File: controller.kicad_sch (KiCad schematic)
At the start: 14 parts, among them J1 Conn_01x06_Female, J2 Conn_01x06_Female, J3 Conn_01x022_Male

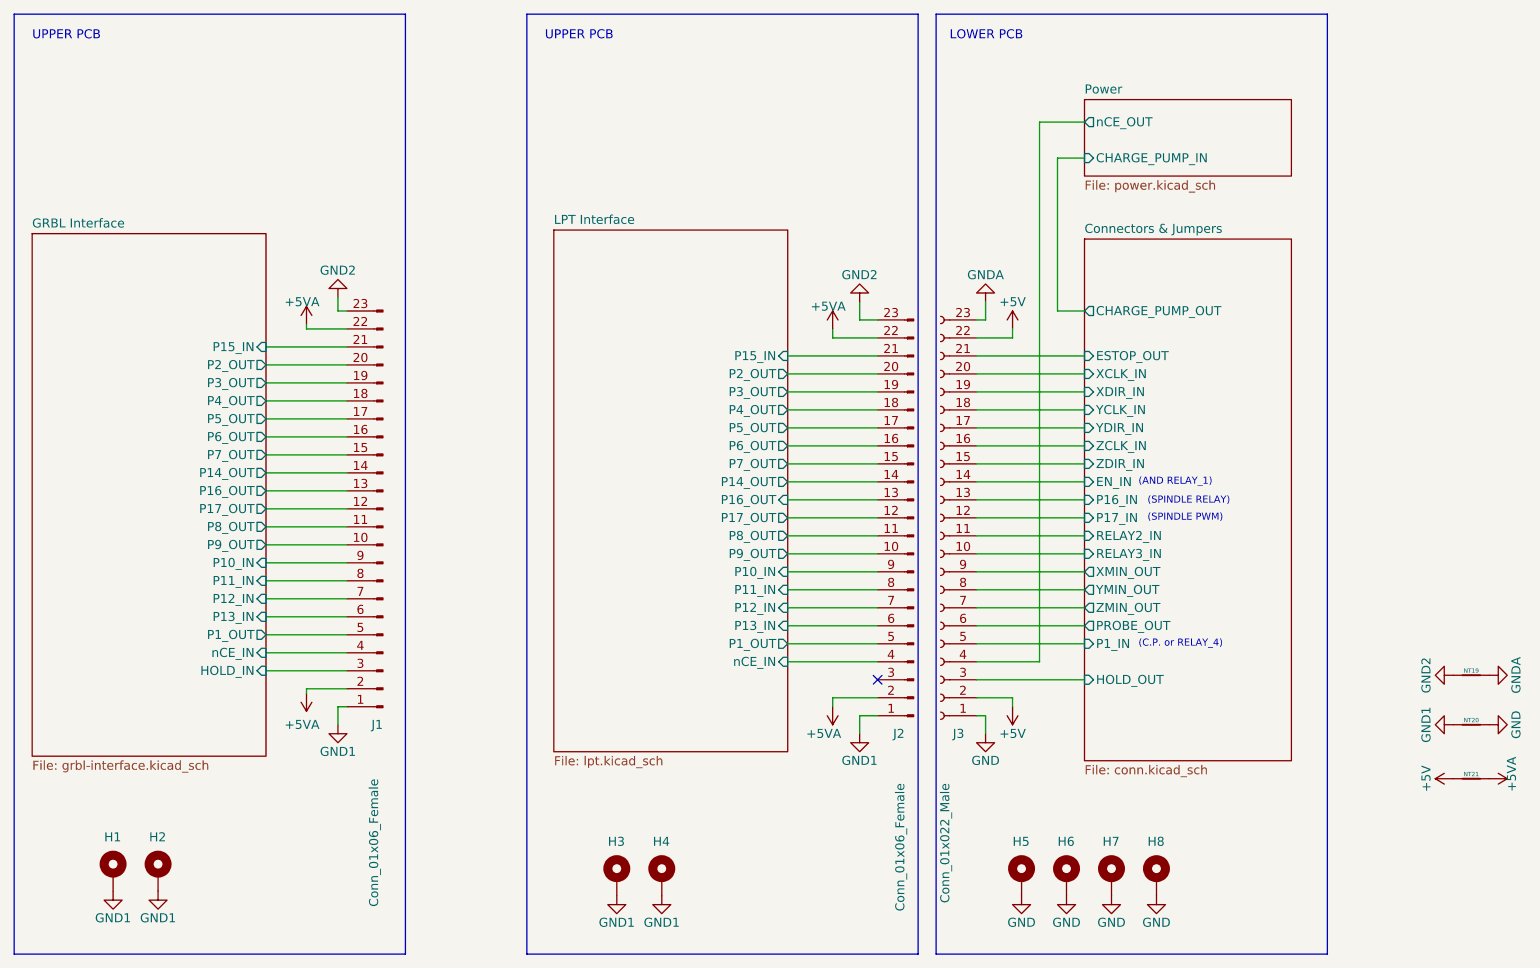
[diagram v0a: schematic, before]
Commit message: GRBL PCB controller work
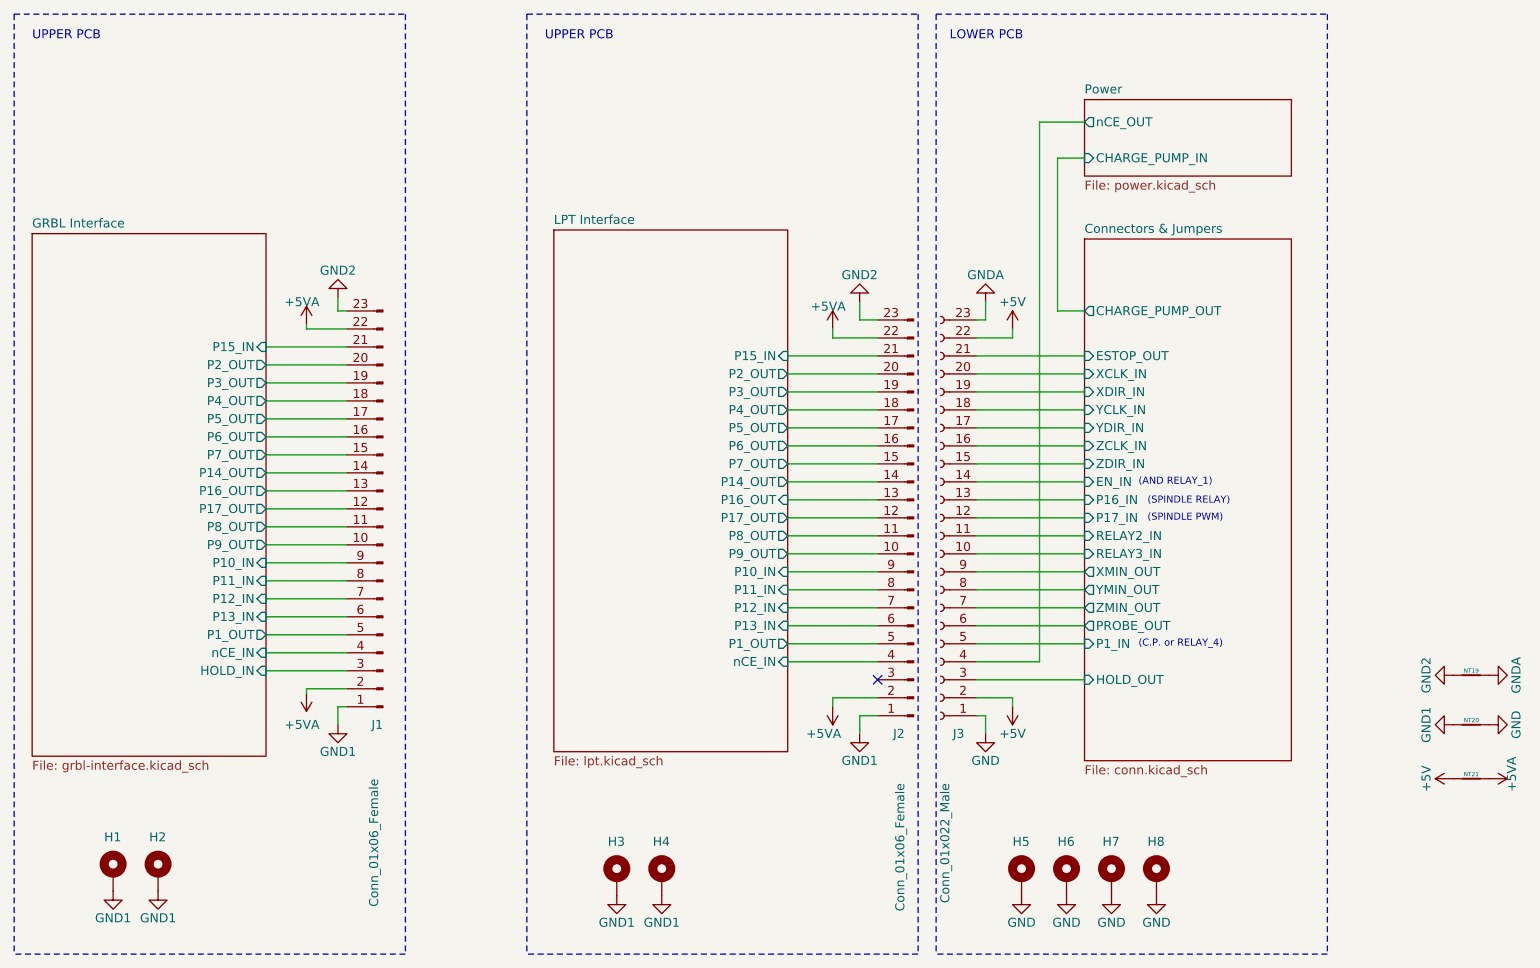
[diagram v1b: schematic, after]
